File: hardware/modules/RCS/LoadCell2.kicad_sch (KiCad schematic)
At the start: 12 parts, among them J101 Conn_01x04, Q101 PNP, U101 HX711

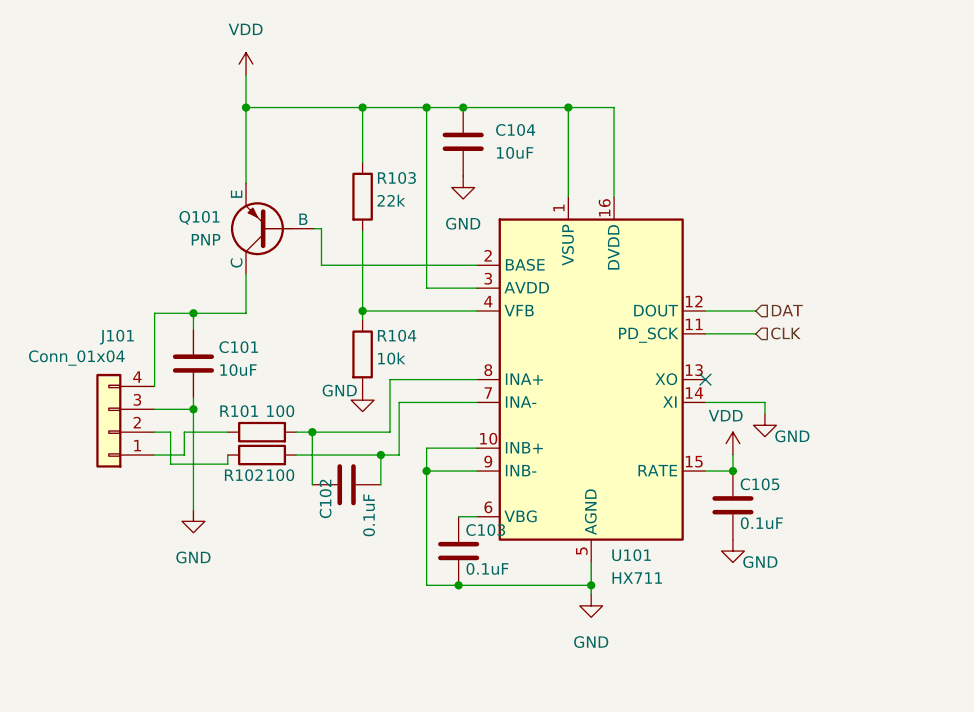
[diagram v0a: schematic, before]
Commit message: RCS回路作成
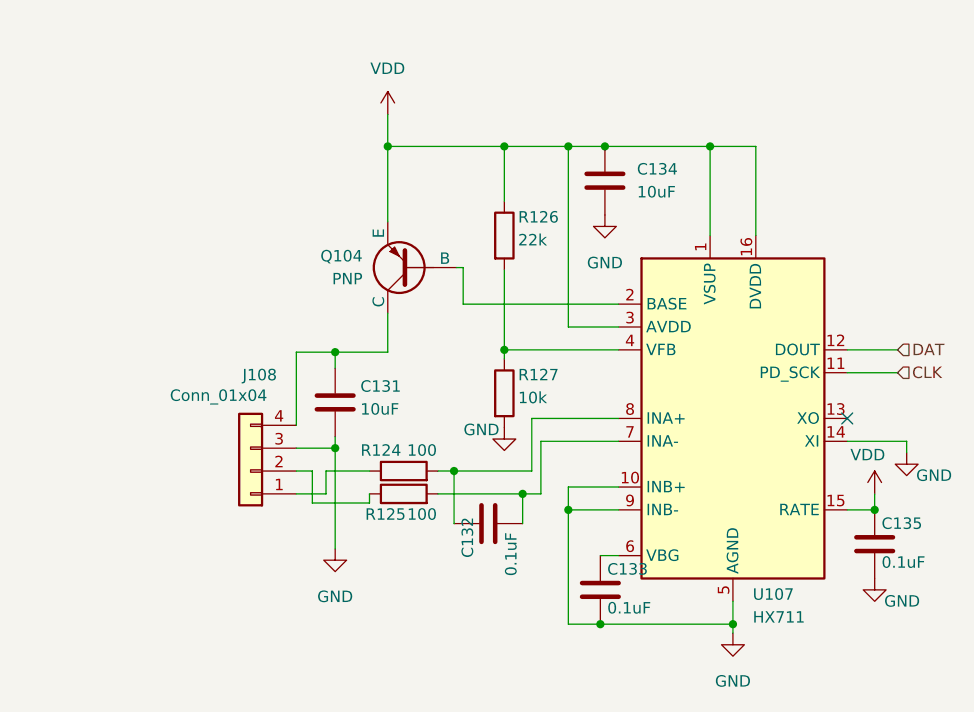
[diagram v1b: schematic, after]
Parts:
- removed C101, C104: 10uF, Capacitor_SMD:C_0603_1608Metric, symbol Device:C
- removed C102, C103, C105: 0.1uF, Capacitor_SMD:C_0402_1005Metric, symbol Device:C
- removed J101: Conn_01x04, Connector_JST:JST_PH_B4B-PH-K_1x04_P2.00mm_Vertical, symbol Connector_Generic:Conn_01x04
- removed Q101: PNP, Package_TO_SOT_SMD:SOT-23, symbol Simulation_SPICE:PNP
- removed R101, R102: 100, Resistor_SMD:R_0402_1005Metric, symbol Device:R
- removed R103: 22k, Resistor_SMD:R_0402_1005Metric, symbol Device:R
- removed R104: 10k, Resistor_SMD:R_0402_1005Metric, symbol Device:R
- removed U101: HX711, Package_SO:SOP-16_3.9x9.9mm_P1.27mm, symbol Analog_ADC:HX711
- added C131, C134: 10uF, Capacitor_SMD:C_0603_1608Metric, symbol Device:C
- added C132, C133, C135: 0.1uF, Capacitor_SMD:C_0402_1005Metric, symbol Device:C
- added J108: Conn_01x04, Connector_JST:JST_PH_B4B-PH-K_1x04_P2.00mm_Vertical, symbol Connector_Generic:Conn_01x04
- added Q104: PNP, Package_TO_SOT_SMD:SOT-23, symbol Simulation_SPICE:PNP
- added R124, R125: 100, Resistor_SMD:R_0402_1005Metric, symbol Device:R
- added R126: 22k, Resistor_SMD:R_0402_1005Metric, symbol Device:R
- added R127: 10k, Resistor_SMD:R_0402_1005Metric, symbol Device:R
- added U107: HX711, Package_SO:SOP-16_3.9x9.9mm_P1.27mm, symbol Analog_ADC:HX711
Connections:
- net CLK: now also U107.11 (PD_SCK)
- net DAT: now also U107.12 (DOUT)
- net GND: now also C131.2, C133.2, C134.2, C135.2, J108.3 (Pin_3), R127.2, U107.10 (INB+), U107.14 (XI), U107.5 (AGND), U107.9 (INB-)
- net VDD: now also C134.1, C135.1, Q104.3 (E), R126.1, U107.1 (VSUP), U107.15 (RATE), U107.16 (DVDD), U107.3 (AVDD)
- new net: Q104.2 (B), U107.2 (BASE)
- new net: R126.2, R127.1, U107.4 (VFB)
- new net: C133.1, U107.6 (VBG)
- new net: C132.2, R125.2, U107.7 (INA-)
- new net: C132.1, R124.2, U107.8 (INA+)
- new net: J108.2 (Pin_2), R125.1
- new net: C131.1, J108.4 (Pin_4), Q104.1 (C)
- new net: J108.1 (Pin_1), R124.1
